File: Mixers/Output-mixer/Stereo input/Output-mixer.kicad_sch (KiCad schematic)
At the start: 123 parts, among them J1 In, J10 In, J11 In, J12 In, J13 Power Input, J14 Conn_01x04_Female, J15 Conn_01x02_Male, J16 Conn_01x04_Male, J17 Conn_01x02_Female, J18 OutR, J19 OutL, J2 In, J20 Jack 3.5 Out, J21 Jack 3.5 Out, J22 OutL, J23 OutR, J3 In, J4 In, J5 In, J6 In, J7 In, J8 In, J9 In, SW1 Mute, SW2 Mute, SW3 Mute, SW4 Mute, SW5 Mute, SW6 Mute, U1 TL072, U2 TL072, U3 TL072, U4 TL072, U6 TL072, U7 TL072, U8 TL072

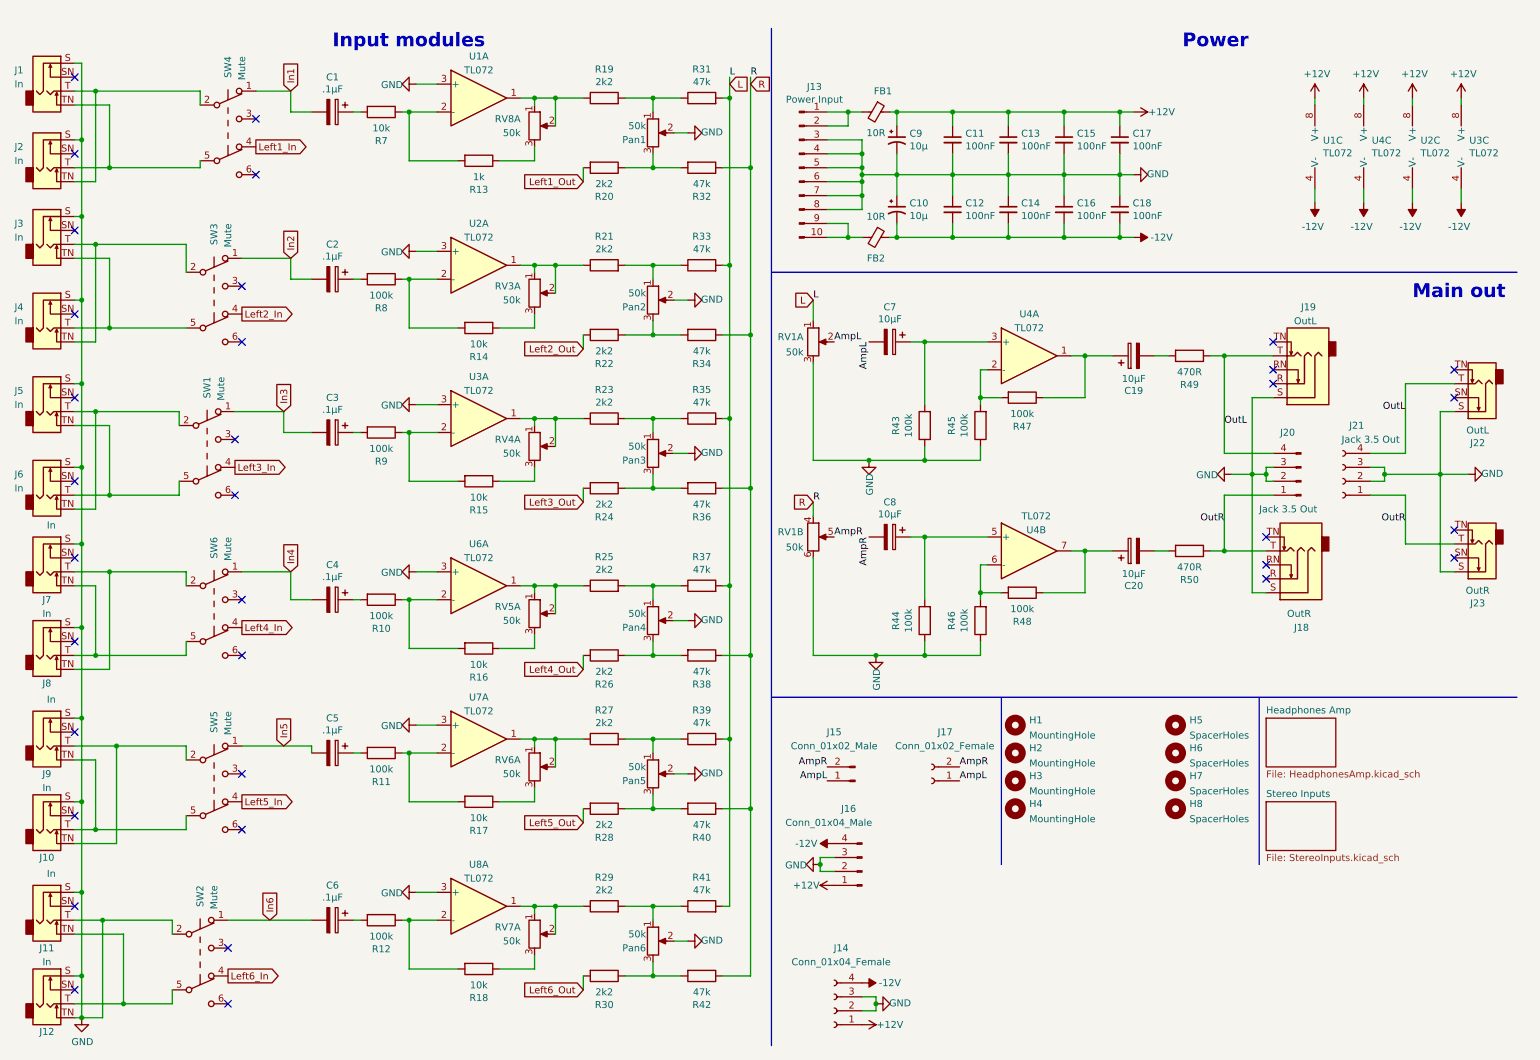
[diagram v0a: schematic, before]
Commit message: update schem (not finished)
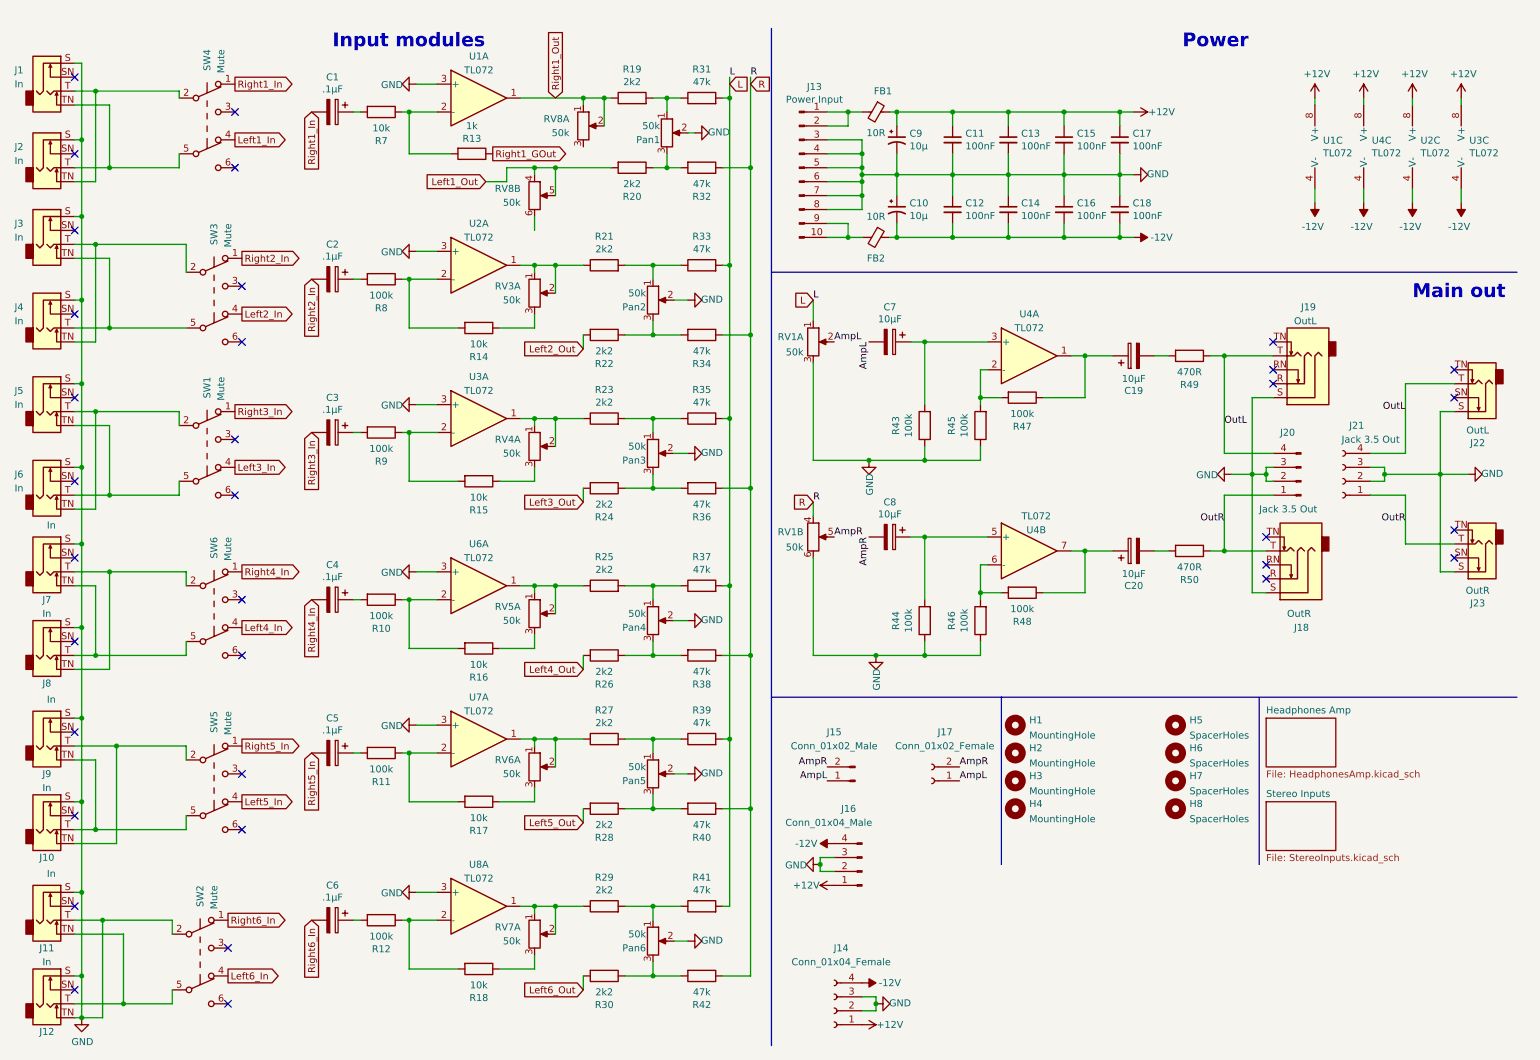
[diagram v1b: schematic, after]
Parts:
- added unit 2 of RV8
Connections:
- net Left1_Out: now also RV8.4, RV8.5
- net at RV8.3: no longer R13.1
- net Right1_Out: now reaches R19.1, RV8.1, RV8.2, U1.1
- net In1 renamed Right1_In
- net In2 renamed Right2_In
- net In3 renamed Right3_In
- net In4 renamed Right4_In
- net In5 renamed Right5_In
- net In6 renamed Right6_In
- new net Right1_GOut: R13.1
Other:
- moved on the sheet: Pan1, R13, R19, R20, RV8A, SW4
